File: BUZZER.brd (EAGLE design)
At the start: 39.8 x 21.5 mm, 8 parts, among them J1 CONECTOR_MACHO, J2 CONECTOR_FEMEA, Q1 BC817, U1 74HC132

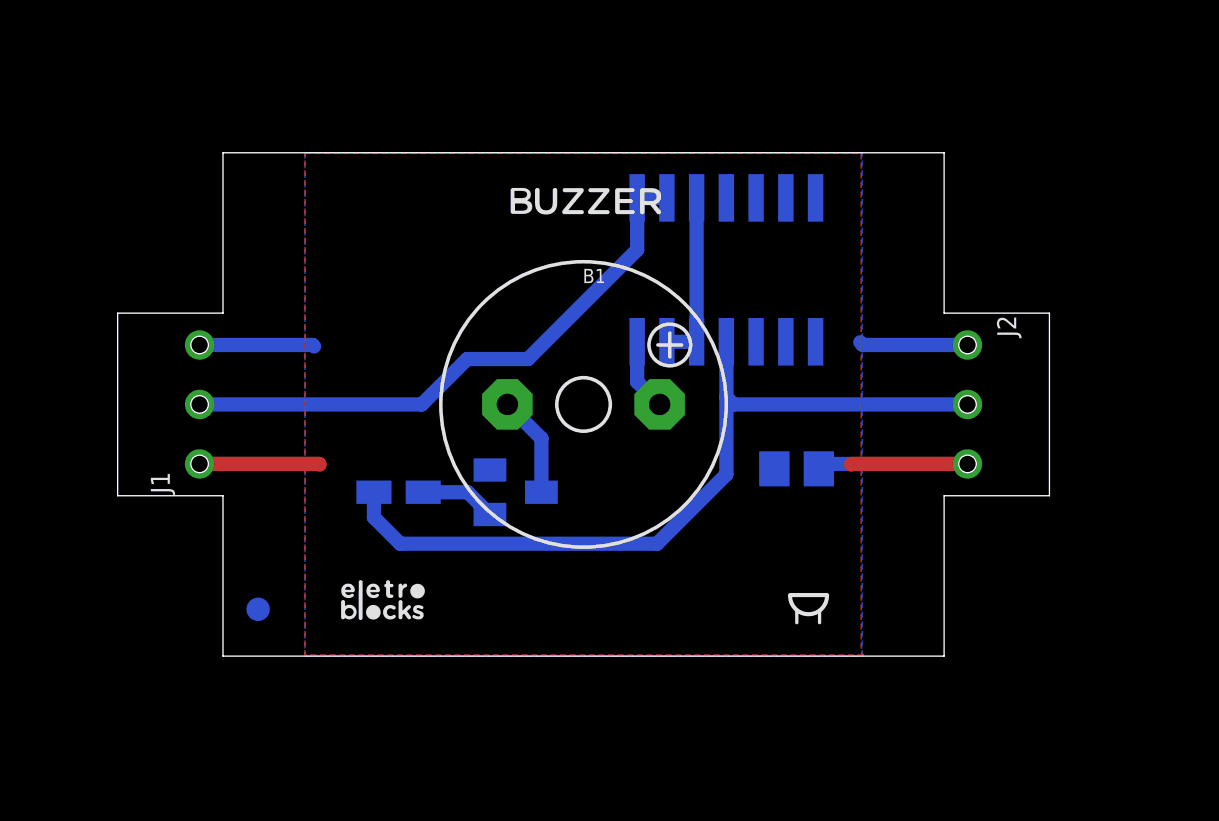
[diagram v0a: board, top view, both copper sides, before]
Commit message: V1.0.3
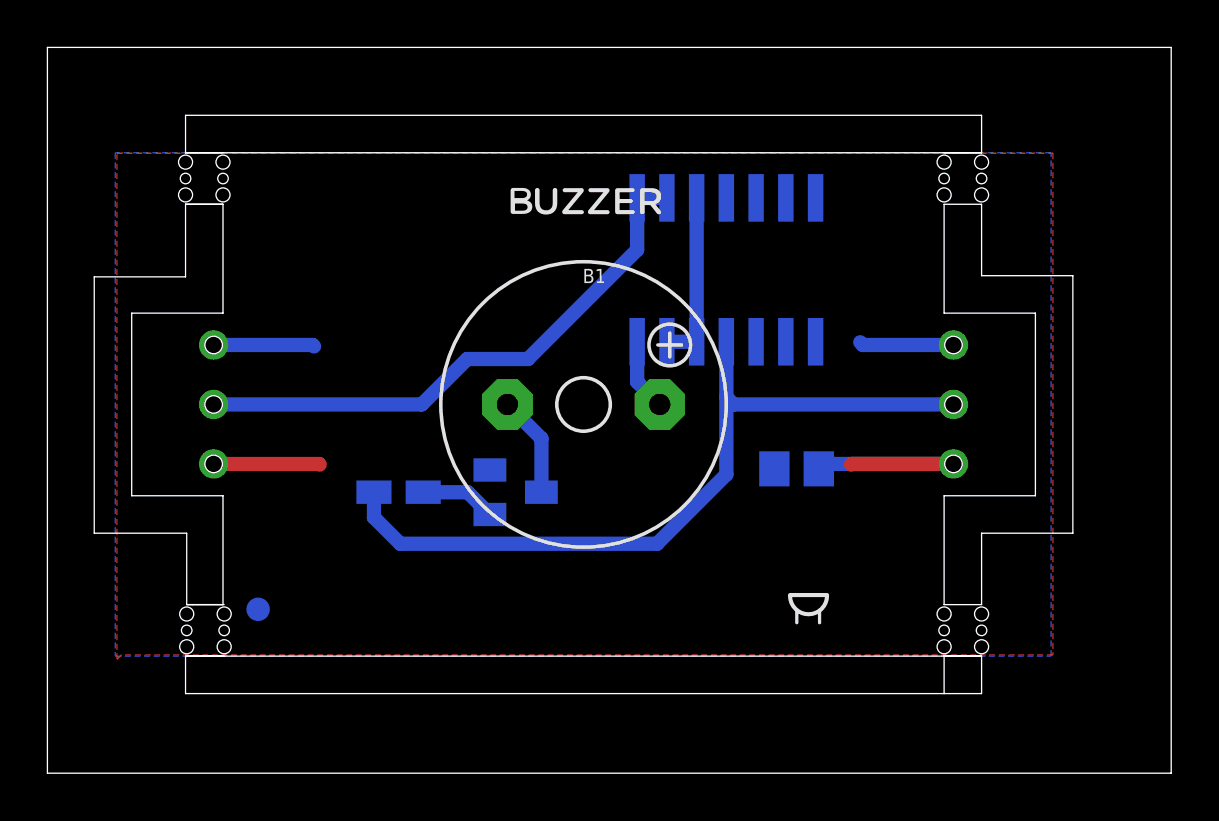
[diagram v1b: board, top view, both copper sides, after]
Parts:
- added U$2, U$3, U$4, U$5: (no value), Eletroblocks Lib:STAMP_DUPLO
- J1: device Eletroblocks Lib:3CONECTOR -> Eletroblocks Lib:MALE
- J2: device Eletroblocks Lib:3CONECTOR -> Eletroblocks Lib:FEMALE
- moved J2 0.60 mm to (27.7, 10.8)
- moved J1 0.60 mm to (-3.90, 10.8)
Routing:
- net VCC: track 19.6 -> 17.8 mm
- net GND: track 9.55 -> 8.35 mm
- net SIGNAL_OUT: track 33.9 -> 33.3 mm
- net SIGNAL_IN: track 24.9 -> 24.3 mm
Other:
- board size 39.8 x 21.5 mm -> 48 x 31 mm
- board text added: "V1.0.3"
- board text removed: "V1.0.1"
